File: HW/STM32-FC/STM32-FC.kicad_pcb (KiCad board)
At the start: 4 copper layers, 38 x 48 mm, 114 parts, among them J1 GH 1.25mm 6P, J10 GH 1.25mm 6P, J11 GH 1.25mm 6P, J12 GH 1.25mm 6P, J13 GH 1.25mm 4P, J14 GH 1.25mm 4P, J15 GH 1.25mm 4P, J2 USB_C_USB2.0_14P, J3 GH 1.25mm 6P, J4 Micro_SD_Card_Det1, J5 JST ZH 1.5mm 2P, J6 PWM_Conn_3x14, J7 ZH 1.5mm 3P, J8 ZH 1.5mm 4P, J9 GH 1.25mm 10P, Q1 S9013, Q2 S9013, SW2 SW_DIP_x03, U1 STM32F407VETx, U10 ATA6561-GBQW, U11 ATA6561-GBQW, U2 USBLC6-2SC6, U3 AMS1117-3.3, U4 AMS1117-3.3, U5 W25X40CLSN, U6 BMI323, U7 ICM-42688-P, U8 LIS2MDLTR, U9 LPS22HH, Y1 16MHz

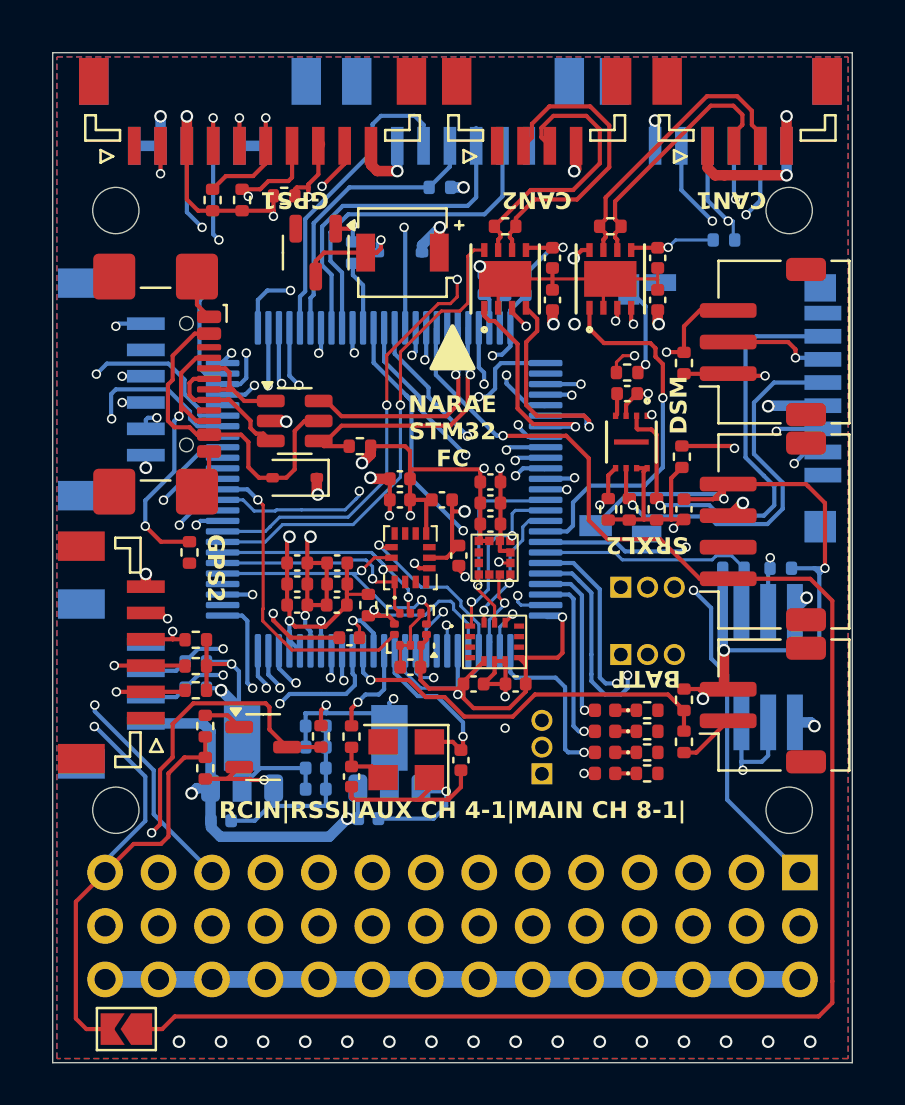
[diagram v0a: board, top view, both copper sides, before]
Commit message: 2025.02.06 PCB routing done v3
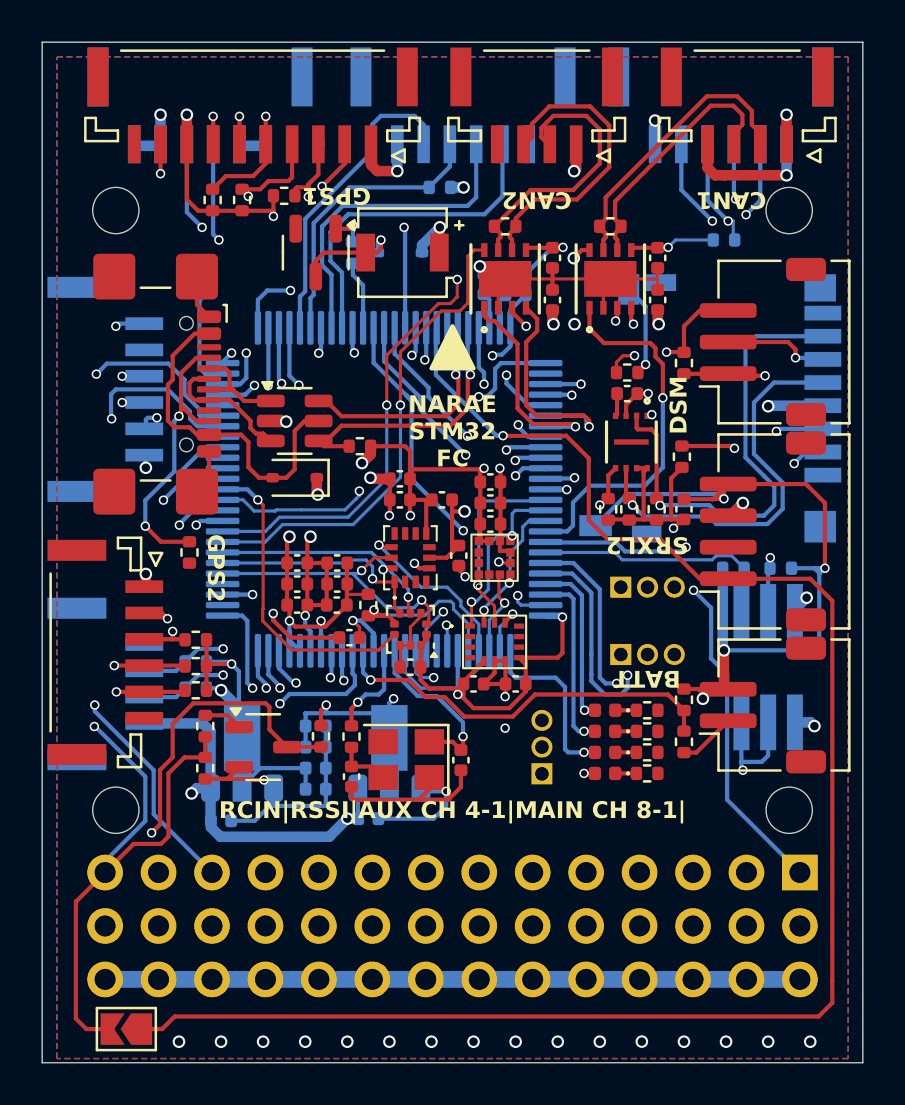
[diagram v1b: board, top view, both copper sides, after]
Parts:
- J1, J10, J11, J12, J3: footprint JST_GH:JST_GH_BM06B-GHS-TBT_06 -> JST_GH:JST_GH_SM06B-GHS-TB_06x1.25mm_Angled
- J13, J14, J15: footprint JST_GH:JST_GH_BM04B-GHS-TBT_04 -> JST_GH:JST_GH_SM04B-GHS-TB_04x1.25mm_Angled
- J9: footprint JST_GH:JST_GH_BM10B-GHS-TBT_10 -> JST_GH:JST_GH_SM10B-GHS-TB_10x1.25mm_Angled
- turned J1 to 90 degrees
- turned J10 to -90 degrees
- turned J11 to 0 degrees
- turned J12 to 0 degrees
- turned J13 to 90 degrees
- turned J14 to 180 degrees
- turned J15 to 180 degrees
- turned J3 to 0 degrees
- turned J9 to 180 degrees
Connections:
- net /TIM4_CH3 renamed /Buzzer
- J1 pad 1: GND -> +3.3V
- J1 pad 2: unconnected-(J1-Pin_2-Pad2) -> /SWDIO
- J1 pad 3: /NRST -> /SWCLK
- J1 pad 4: /SWCLK -> /NRST
- J1 pad 5: /SWDIO -> unconnected-(J1-Pin_5-Pad5)
- J1 pad 6: +3.3V -> GND
- J10 pad 1: GND -> +5V
- J10 pad 2: /I2C2_SDA -> /UART5_TX
- J10 pad 3: /I2C2_SCL -> /UART5_RX
- J10 pad 4: /UART5_RX -> /I2C2_SCL
- J10 pad 5: /UART5_TX -> /I2C2_SDA
- J10 pad 6: +5V -> GND
- J11 pad 1: GND -> +5V
- J11 pad 2: /UART2_RTS -> /UART2_TX
- J11 pad 3: /UART2_CTS -> /UART2_RX
- J11 pad 4: /UART2_RX -> /UART2_CTS
- J11 pad 5: /UART2_TX -> /UART2_RTS
- J11 pad 6: +5V -> GND
- J12 pad 1: GND -> +5V
- J12 pad 2: /UART3_RTS -> /UART3_TX
- J12 pad 3: /UART3_CTS -> /UART3_RX
- J12 pad 4: /UART3_RX -> /UART3_CTS
- J12 pad 5: /UART3_TX -> /UART3_RTS
- J12 pad 6: +5V -> GND
- J13 pad 1: GND -> +5V
- J13 pad 2: /I2C1_SDA -> /I2C1_SCL
- J13 pad 3: /I2C1_SCL -> /I2C1_SDA
- J13 pad 4: +5V -> GND
- J14 pad 1: GND -> +5V
- J14 pad 2: /Communication/CAN1_N -> /Communication/CAN1_P
- J14 pad 3: /Communication/CAN1_P -> /Communication/CAN1_N
- J14 pad 4: +5V -> GND
- J15 pad 1: GND -> +5V
- J15 pad 2: /Communication/CAN2_N -> /Communication/CAN2_P
- J15 pad 3: /Communication/CAN2_P -> /Communication/CAN2_N
- J15 pad 4: +5V -> GND
- J3 pad 1: GND -> +5V
- J3 pad 2: GND -> +5V
- J3 pad 3: /PM_VOLTAGE -> /PM_CURRENT
- J3 pad 4: /PM_CURRENT -> /PM_VOLTAGE
- J3 pad 5: +5V -> GND
- J3 pad 6: +5V -> GND
- J9 pad 1: GND -> +5V
- J9 pad 10: +5V -> GND
- J9 pad 2: /GPS1_BUZZER -> /UART4_TX
- J9 pad 3: +3.3V -> /UART4_RX
- J9 pad 4: /GPS1_SW_LED -> /I2C3_SCL
- J9 pad 5: /GPS1_SW -> /I2C3_SDA
- J9 pad 6: /I2C3_SDA -> /GPS1_SW
- J9 pad 7: /I2C3_SCL -> /GPS1_SW_LED
- J9 pad 8: /UART4_RX -> +3.3V
- J9 pad 9: /UART4_TX -> /GPS1_BUZZER
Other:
- board size 38 x 48 mm -> 39 x 48.5 mm
